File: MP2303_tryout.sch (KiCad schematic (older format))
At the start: 16 parts, among them J1 INPUT, J2 OUTPUT_3V3, U1 MP2303A_ALT

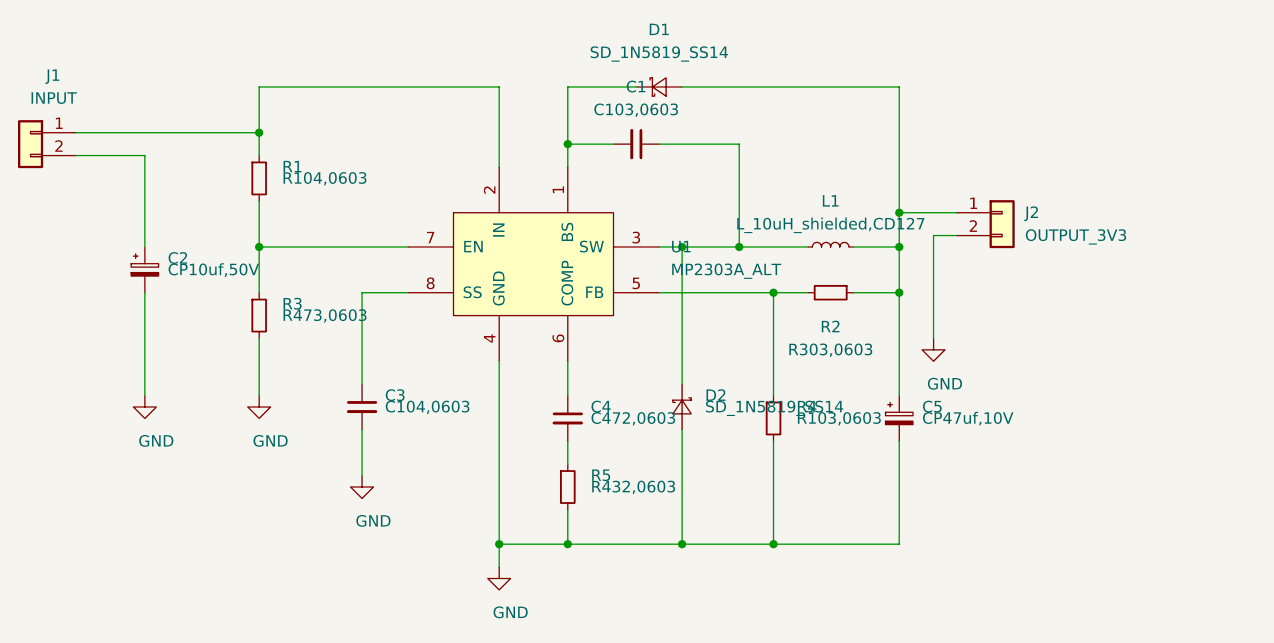
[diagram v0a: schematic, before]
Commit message: update,
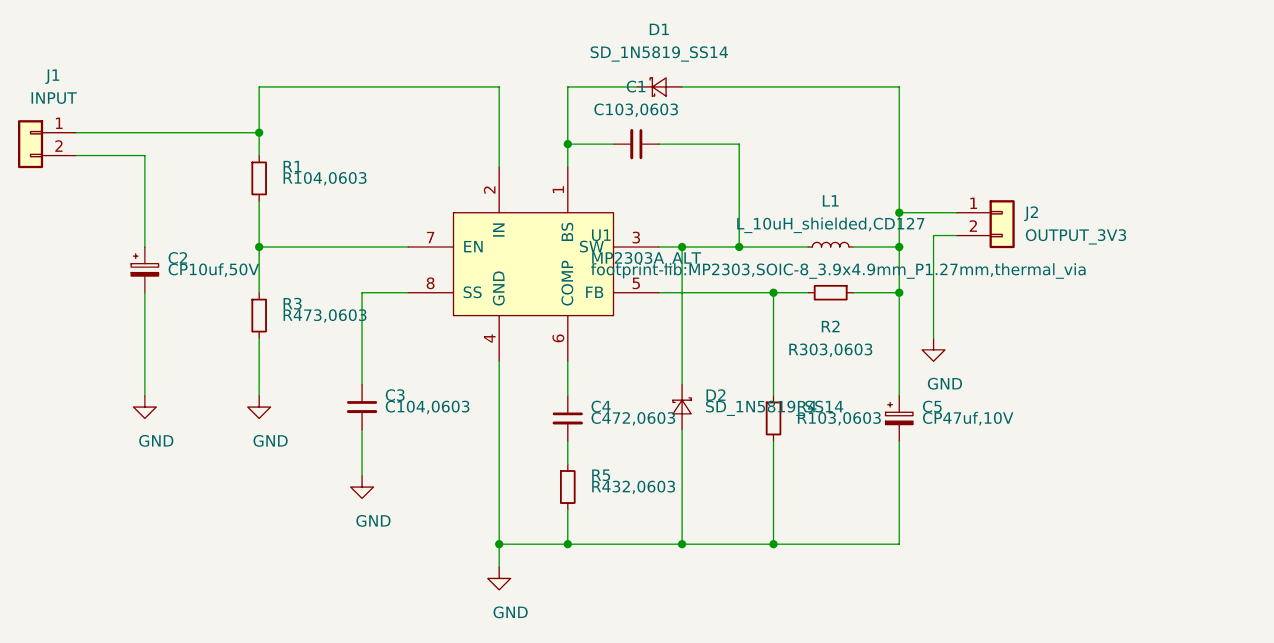
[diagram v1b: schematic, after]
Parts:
- U1: footprint Package_SO:SOIC-8_3.9x4.9mm_P1.27mm -> footprint-lib:MP2303,SOIC-8_3.9x4.9mm_P1.27mm,thermal_via
